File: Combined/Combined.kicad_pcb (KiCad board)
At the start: 2 copper layers, 109.5 x 100.3 mm, 38 parts, among them J1 motor, J2 230V_IN, J3 Home_Controller, J4 Open_Close_Sensor, J5 Extras, K1 SANYOU_SRD_Form_C, K2 SANYOU_SRD_Form_C, Q1 BC547, Q2 BC547, U1 Vcc_one_supply, U2 ATmega328P-PU, U3 Current_Transformer, U4 LM741, Y1 Crystal

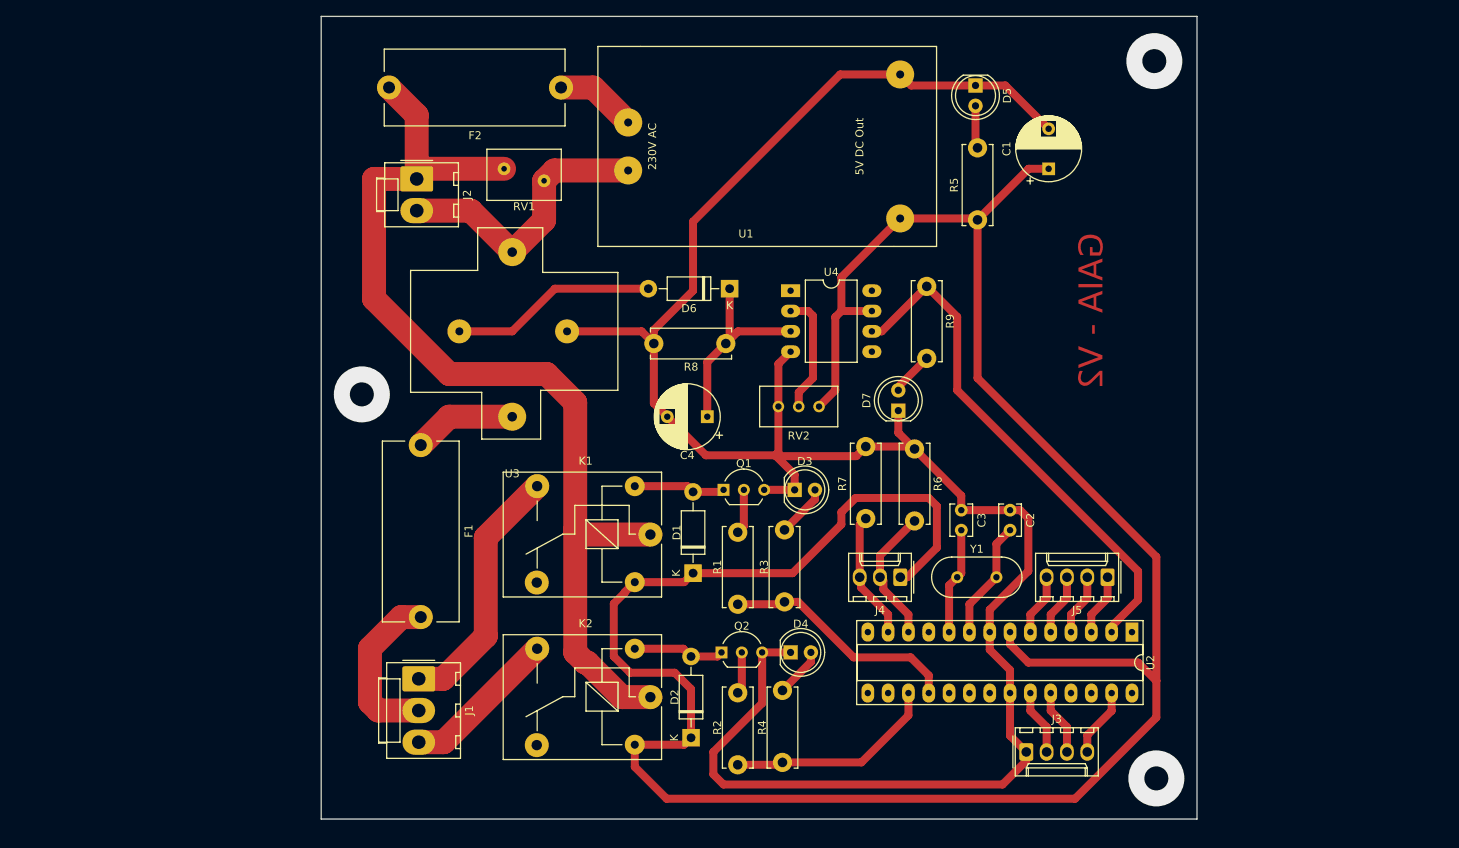
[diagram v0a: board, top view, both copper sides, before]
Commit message: working PCB v2
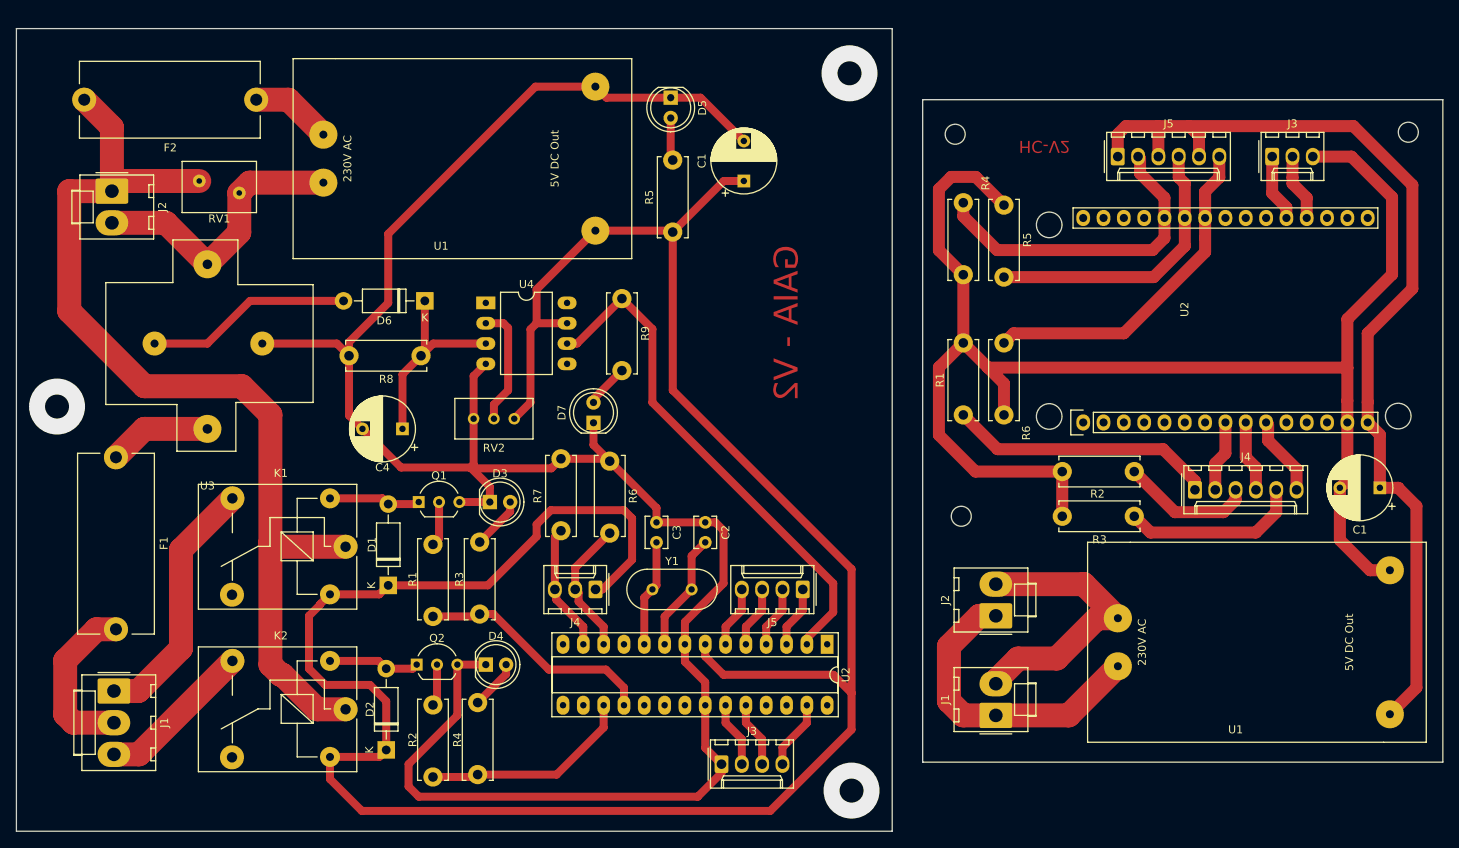
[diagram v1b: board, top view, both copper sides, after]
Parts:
- added  : H, MountingHole:MountingHole_2.5mm, F.Cu at (160.0, 96.3)
- added  : H, MountingHole:MountingHole_2.5mm, F.Cu at (215.9, 48.3)
- added  : H, MountingHole:MountingHole_2.5mm, F.Cu at (159.3, 48.5)
- added C1: CP1, Capacitor_THT:CP_Radial_D8.0mm_P5.00mm, F.Cu at (212.3, 92.7)
- added J1: supply, Connector_Molex:Molex_KK-396_A-41791-0002_1x02_P3.96mm_Vertical, F.Cu at (164.3, 121.2)
- added J2: motor, Connector_Molex:Molex_KK-396_A-41791-0002_1x02_P3.96mm_Vertical, F.Cu at (164.3, 108.7)
- added J3: Conn_01x03, Connector_Molex:Molex_KK-254_AE-6410-03A_1x03_P2.54mm_Vertical, F.Cu at (198.9, 51.3)
- added J4: LED_ARRAY, Connector_Molex:Molex_KK-254_AE-6410-06A_1x06_P2.54mm_Vertical, F.Cu at (189.2, 93.0)
- added J5: SWITCH_ARRAY, Connector_Molex:Molex_KK-254_AE-6410-06A_1x06_P2.54mm_Vertical, F.Cu at (179.6, 51.3)
- added R1: 330E, gaia_gate:resistor, F.Cu at (160.3, 85.6)
- added R2: 330E, gaia_gate:resistor, F.Cu at (183.6, 90.7)
- added R3: 330E, gaia_gate:resistor, F.Cu at (183.6, 96.3)
- added R4: 10K, gaia_gate:resistor, F.Cu at (160.3, 68.1)
- added R5: 10K, gaia_gate:resistor, F.Cu at (165.4, 55.4)
- added R6: 10K, gaia_gate:resistor, F.Cu at (165.4, 85.6)
- added U1: pcb_power_supply_Vcc_one_supply, gaia_gate:230_5V_supply_HiLink, F.Cu at (196.6, 112.0)
- added U2: NodeMCU, gaia-gate:NodeMCU, F.Cu at (175.3, 81.8)
- moved C2 38.1 mm to (128.0, 97.0)
- moved C3 38.1 mm to (121.9, 97.0)
- moved C4 38.1 mm to (90.2, 85.3)
- moved D1 38.1 mm to (88.4, 104.9)
- moved D3 38.1 mm to (101.1, 94.5)
- moved D5 38.1 mm to (123.7, 43.9)
- moved J4 38.1 mm to (114.3, 105.4)
- moved Q2 38.1 mm to (91.9, 114.8)
- moved R1 38.1 mm to (94.0, 97.8)
- moved R2 38.1 mm to (94.0, 117.9)
- moved R4 38.1 mm to (99.6, 130.6)
- moved RV1 38.1 mm to (64.8, 54.4)
- moved U1 38.1 mm to (97.3, 51.6)
- moved F1 38.1 mm to (54.4, 88.4)
- moved J1 38.1 mm to (54.1, 118.1)
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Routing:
- net GND: track 270.8 -> 459.7 mm
- net +5V: track 309.7 -> 434.6 mm
- net Net-(J5-Pad6): track 0.00 -> 42.5 mm
- net Net-(J5-Pad2): track 7.70 -> 48.5 mm
- net Net-(J1-Pad1): track 32.0 -> 70.7 mm
- net Net-(J1-Pad2): track 0.00 -> 35.9 mm
- net Net-(J5-Pad4): track 7.70 -> 43.4 mm
- net Net-(J4-Pad1): track 0.00 -> 33.5 mm
- net Net-(J4-Pad5): track 0.00 -> 22.4 mm
- net Net-(J4-Pad3): track 16.0 -> 32.7 mm
- net Net-(J4-Pad6): track 0.00 -> 10.0 mm
- net Net-(J4-Pad2): track 17.2 -> 26.1 mm
- net Net-(J4-Pad4): track 0.00 -> 8.95 mm
- net Net-(J3-Pad1): track 0.00 -> 8.41 mm
- net Net-(J3-Pad2): track 8.21 -> 16.6 mm
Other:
- board size 109.5 x 100.3 mm -> 178.3 x 100.3 mm
- board text added: "HC-V2"
